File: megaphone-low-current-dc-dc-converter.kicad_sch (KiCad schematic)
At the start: 9 parts, among them U1 TPS631000DRLR

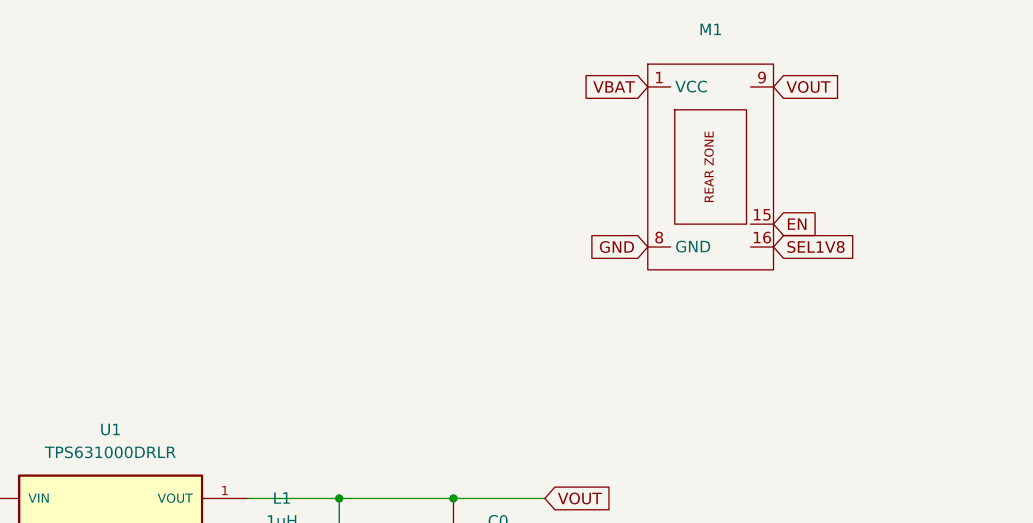
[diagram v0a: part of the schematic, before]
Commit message: finish PCB layout
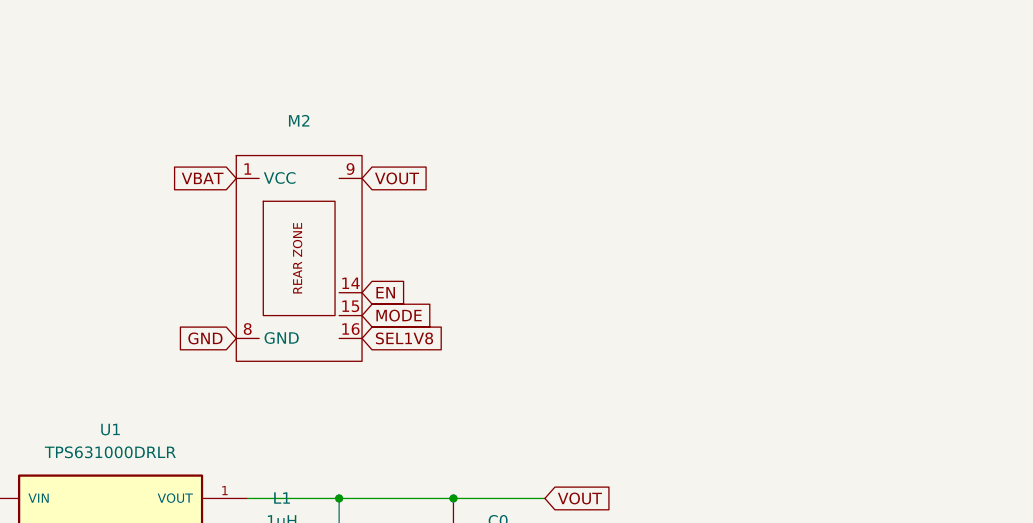
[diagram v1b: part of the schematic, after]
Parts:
- removed M1: ~, MegaCastle:MegaCastle2x8-Module-I7.0x15.5-M8183-PANEL-NIBBLE, symbol MegaCastle:MegaCastle2x8-Module-I7.0x15.5-M8183
- added M2: ~, MegaCastle:MegaCastle2x8-Module-I7.0x15.5-M8187-PANEL-NIBBLE, symbol MegaCastle:MegaCastle2x8-Module-I7.0x15.5-M8187
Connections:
- net EN: now also M2.14
- net GND: now also M2.8 (GND)
- net MODE: now also M2.15
- net SEL1V8: now also M2.16
- net VBAT: now also M2.1 (VCC)
- net VOUT: now also M2.9
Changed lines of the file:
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@@
 	(global_label "SEL1V8"
 		(shape input)
-		(at 138.43 63.5 0)
+		(at 92.71 73.66 0)
 		(fields_autoplaced yes)
 		(effects
@@
 		)
 		(property "Intersheetrefs" "${INTERSHEET_REFS}"
-			(at 148.3094 63.5 0)
+			(at 102.5894 73.66 0)
 			(effects
 				(font
@@
 	(global_label "VBAT"
 		(shape input)
-		(at 124.46 45.72 180)
+		(at 78.74 55.88 180)
 		(fields_autoplaced yes)
 		(effects
@@
 		)
 		(property "Intersheetrefs" "${INTERSHEET_REFS}"
-			(at 117.06 45.72 0)
+			(at 71.34 55.88 0)
 			(effects
 				(font
@@
 	(global_label "EN"
 		(shape input)
-		(at 138.43 60.96 0)
+		(at 92.71 68.58 0)
 		(fields_autoplaced yes)
 		(effects
@@
 		)
 		(property "Intersheetrefs" "${INTERSHEET_REFS}"
-			(at 143.8947 60.96 0)
+			(at 98.1747 68.58 0)
 			(effects
 				(font
@@
 	(global_label "VOUT"
 		(shape input)
-		(at 138.43 45.72 0)
+		(at 92.71 55.88 0)
 		(fields_autoplaced yes)
 		(effects
@@
 		)
 		(property "Intersheetrefs" "${INTERSHEET_REFS}"
-			(at 146.1324 45.72 0)
+			(at 100.4124 55.88 0)
 			(effects
 				(font
@@
 	(global_label "GND"
 		(shape input)
-		(at 124.46 63.5 180)
+		(at 78.74 73.66 180)
 		(fields_autoplaced yes)
 		(effects
@@
 		)
 		(property "Intersheetrefs" "${INTERSHEET_REFS}"
-			(at 117.6043 63.5 0)
+			(at 71.8843 73.66 0)
 			(effects
 				(font
@@
 		(property "Intersheetrefs" "${INTERSHEET_REFS}"
 			(at 120.7324 91.44 0)
+			(effects
+				(font
+					(size 1.27 1.27)
+				)
+				(justify left)
+				(hide yes)
+			)
+		)
+	)
+	(global_label "MODE"
+		(shape input)
+		(at 92.71 71.12 0)
+		(fields_autoplaced yes)
+		(effects
+			(font
+				(size 1.27 1.27)
+			)
+			(justify left)
+		)
+		(property "Intersheetrefs" "${INTERSHEET_REFS}"
+			(at 100.8961 71.12 0)
 			(effects
 				(font
@@
 	)
 	(symbol
+		(lib_id "MegaCastle:MegaCastle2x8-Module-I7.0x15.5-M8187")
+		(at 85.09 64.77 0)
+		(unit 1)
+		(exclude_from_sim no)
+		(in_bom yes)
+		(on_board yes)
+		(dnp no)
+		(fields_autoplaced yes)
+		(property "Reference" "M2"
+			(at 85.725 49.53 0)
+			(effects
+				(font
+					(size 1.27 1.27)
+				)
+			)
+		)
+		(property "Value" "~"
+			(at 85.725 52.07 0)
+			(effects
+				(font
+					(size 1.27 1.27)
+				)
+			)
+		)
+		(property "Footprint" "MegaCastle:MegaCastle2x8-Module-I7.0x15.5-M8187-PANEL-NIBBLE"
+			(at 85.09 81.28 0)
+			(effects
+				(font
+					(size 1.27 1.27)
+				)
+				(hide yes)
+			)
+		)
+		(property "Datasheet" ""
+			(at 85.09 59.69 0)
+			(effects
+				(font
+					(size 1.27 1.27)
+				)
+				(hide yes)
+			)
+		)
+		(property "Description" "Generated using footprint-gen .. 7 14 6 M8187"
+			(at 85.09 64.77 0)
+			(effects
+				(font
+					(size 1.27 1.27)
+				)
+				(hide yes)
+			)
+		)
+		(pin "14"
+		)
+		(pin "16"
+		)
+		(pin "8"
+		)
+		(pin "1"
+		)
+		(pin "15"
+		)
+		(pin "9"
+		)
+		(instances
+			(project ""
+				(path "/6fccb5b0-46ff-4014-9169-aa61e4064f3f"
+					(reference "M2")
+					(unit 1)
+				)
+			)
+		)
+	)
+	(symbol
 		(lib_id "power:Earth")
 		(at 80.01 109.22 0)
@@
 					(unit 1)
 				)
-			)
-		)
-	)
-	(symbol
-		(lib_id "MegaCastle:MegaCastle2x8-Module-I7.0x15.5-M8183")
-		(at 130.81 54.61 0)
-		(unit 1)
-		(exclude_from_sim no)
-		(in_bom yes)
-		(on_board yes)
-		(dnp no)
-		(fields_autoplaced yes)
-		(property "Reference" "M1"
-			(at 131.445 39.37 0)
-			(effects
-				(font
-					(size 1.27 1.27)
-				)
-			)
-		)
-		(property "Value" "~"
-			(at 131.445 41.91 0)
-			(effects
-				(font
-					(size 1.27 1.27)
-				)
-			)
-		)
-		(property "Footprint" "MegaCastle:MegaCastle2x8-Module-I7.0x15.5-M8183-PANEL-NIBBLE"
-			(at 130.81 71.12 0)
-			(effects
-				(font
-					(size 1.27 1.27)
-				)
-				(hide yes)
-			)
-		)
-		(property "Datasheet" ""
-			(at 130.81 49.53 0)
-			(effects
-				(font
-					(size 1.27 1.27)
-				)
-				(hide yes)
-			)
-		)
-		(property "Description" "Generated using footprint-gen .. 7 14 5 M8183"
-			(at 130.81 54.61 0)
-			(effects
-				(font
-					(size 1.27 1.27)
-				)
-				(hide yes)
-			)
-		)
-		(pin "1"
-		)
-		(pin "8"
-		)
-		(pin "9"
-		)
-		(pin "16"
-		)
-		(pin "15"
-		)
-		(instances
-			(project ""
-				(path "/6fccb5b0-46ff-4014-9169-aa61e4064f3f"
-					(reference "M1")
-					(unit 1)
-				)
